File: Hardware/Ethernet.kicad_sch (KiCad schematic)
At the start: 31 parts, among them J5 MagJack_PoE, U4 KSZ8041NL/I

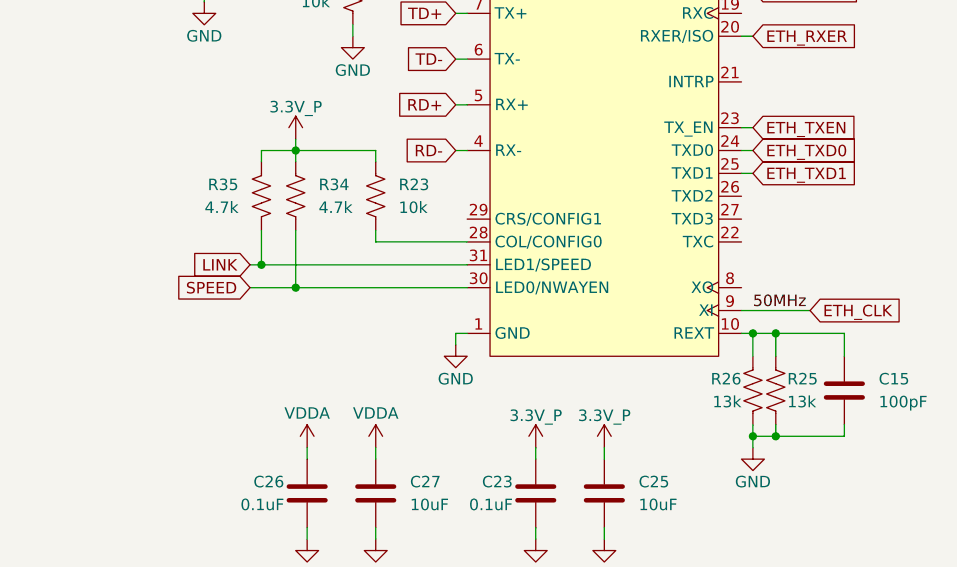
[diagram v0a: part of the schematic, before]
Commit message: More WIP
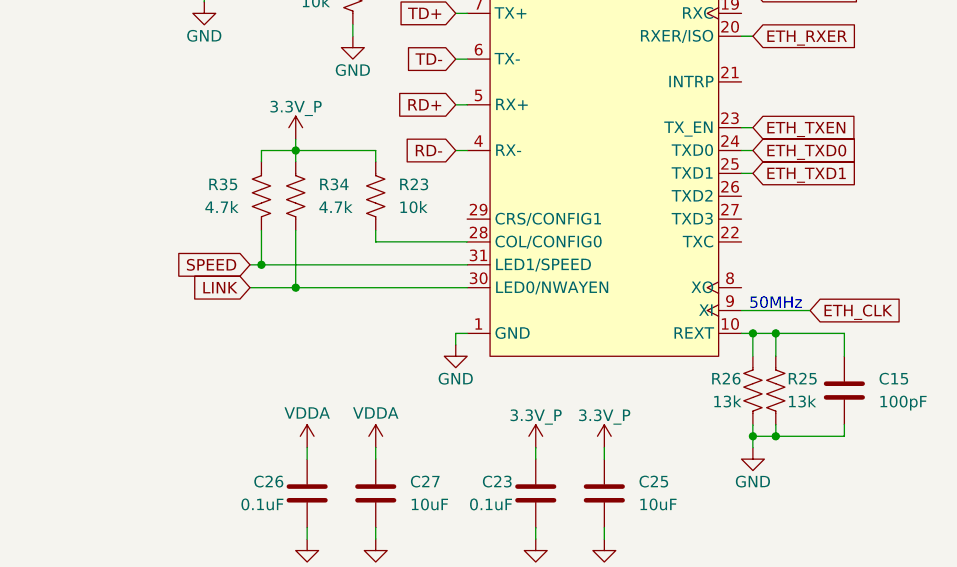
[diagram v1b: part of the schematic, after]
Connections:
- net LINK: now also R34.2, U4.30 (LED0/NWAYEN); no longer R35.2, U4.31 (LED1/SPEED)
- net SPEED: now also R35.2, U4.31 (LED1/SPEED); no longer R34.2, U4.30 (LED0/NWAYEN)
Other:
- note added: "50MHz"
